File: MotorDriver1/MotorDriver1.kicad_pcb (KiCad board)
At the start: 2 copper layers, 74 parts, among them IC1 STM32C092RCT6, J1 GT-USB-7010ASV, J2 Conn_01x02, J3 Conn_01x02, Q1 IRLZ44NSTRLPBF, Q2 IRLZ44NSTRLPBF, Q3 IRLZ44NSTRLPBF, Q4 IRLZ44NSTRLPBF, SW1 K2-6639SP-C4SC-04, SW2 K2-6639SP-C4SC-04, SW3 K2-6639SP-C4SC-04, U1 TPS22916CNYFPR, U2 CH340X, U3 XIAO-ESP32-C5-DIP, U4 MCP2562FDT-H/SN, U5 MCP2562FDT-H/SN, U7 LMV358AIDR, Y1 48 MHz, Y2 32.768 kHz

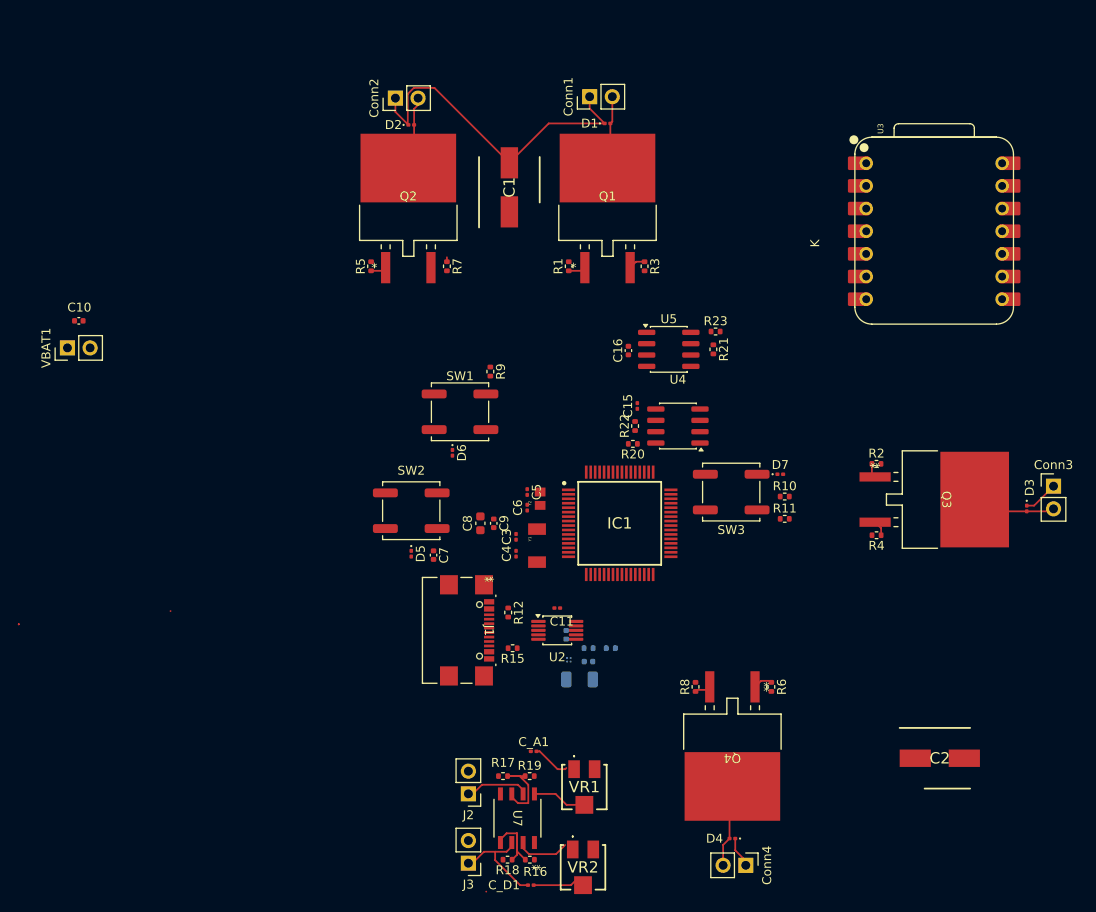
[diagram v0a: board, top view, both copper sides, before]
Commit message: Exported final JLCPCB files
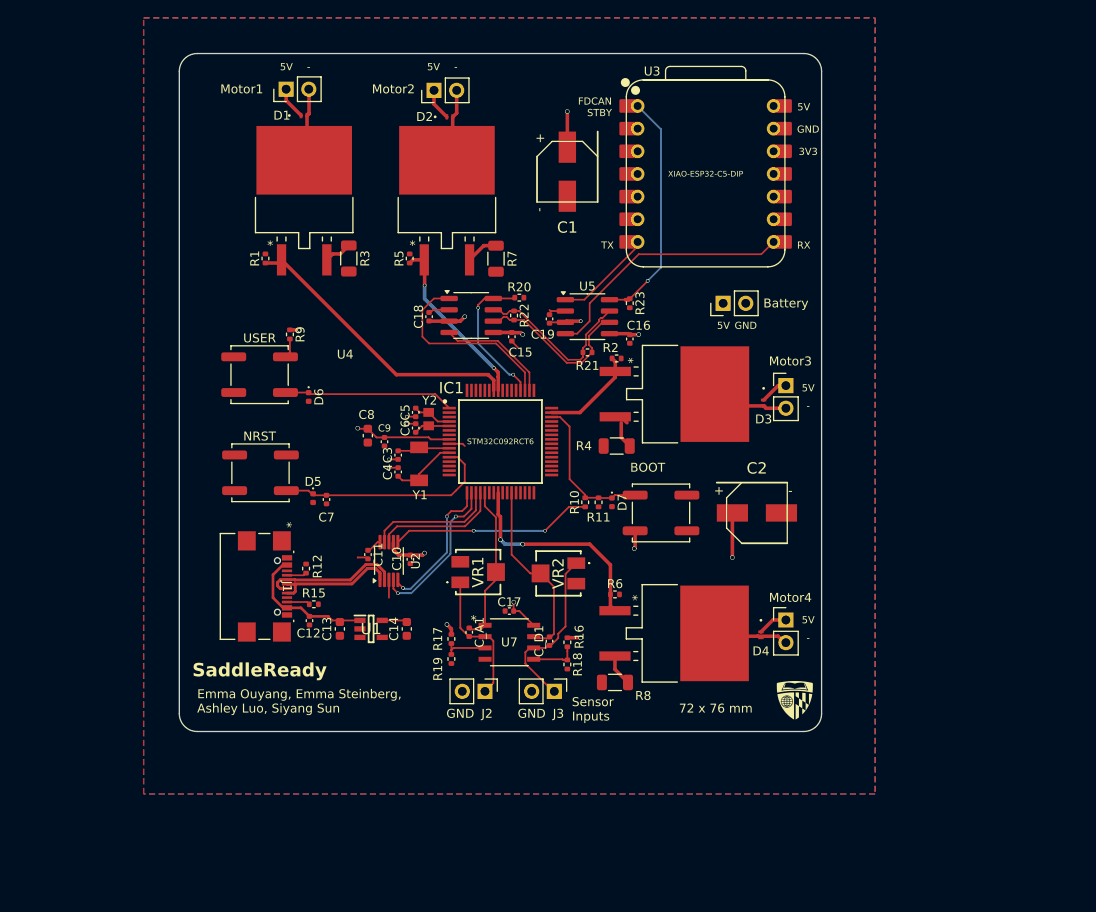
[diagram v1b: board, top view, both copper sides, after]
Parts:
- removed R13, R14: 10k, 1%, Resistor_SMD:R_0402_1005Metric
- added C17: 100 nF, Capacitor_SMD:C_0402_1005Metric, F.Cu at (153.0, 112.5)
- added C18: 100 nF, Capacitor_SMD:C_0402_1005Metric, F.Cu at (144.0, 79.5)
- added C19: 100 nF, Capacitor_SMD:C_0402_1005Metric, F.Cu at (157.5, 79.8)
- added G***: LOGO, LOGO, F.Cu at (185.0, 122.5)
- C10, C16: value 100nF -> 100 nF
- C11, C5, C6: footprint Capacitor_SMD:C_0201_0603Metric -> Capacitor_SMD:C_0402_1005Metric
- C12: value 100nF -> 100 nF; moved to F.Cu
- C13: value 100nF -> 1 uF; footprint Capacitor_SMD:C_0402_1005Metric -> Capacitor_SMD:C_0603_1608Metric; moved to F.Cu
- C14: value 10uF -> 1 uF; footprint Capacitor_SMD:C_1206_3216Metric -> Capacitor_SMD:C_0603_1608Metric; moved to F.Cu
- C15: value 100nF -> 100 nF; footprint Capacitor_SMD:C_0201_0603Metric -> Capacitor_SMD:C_0402_1005Metric
- C3, C4: value 8 pF -> 8 pF, 0.1%; footprint Capacitor_SMD:C_0201_0603Metric -> Capacitor_SMD:C_0402_1005Metric
- C_A1, C_D1: value 44nF -> 47 nF; footprint Capacitor_SMD:C_0201_0603Metric -> Capacitor_SMD:C_0402_1005Metric
- D1, D2, D3, D4: value Power_D -> SM5819L2-TP; footprint Diode_SMD:D_0201_0603Metric -> footprintLib:SDO_SM5819L2-TP_MCE
- D5, D6, D7: value ESDALC6V1-1U2 -> ESDALC6V1-1M2; footprint Diode_SMD:D_0201_0603Metric -> Diode_SMD:D_0402_1005Metric
- R1, R16, R17, R2, R5, R6: value 10000 -> 10k
- R18, R19: value 1800 -> 1.8k
- R3, R4, R7, R8: footprint Resistor_SMD:R_0402_1005Metric -> Resistor_SMD:R_1206_3216Metric
- U1: value TPS22916CNYFPR -> NCP361SNT1G; footprint footprintLib:TPS22916CNYFPR -> footprintLib:SOT95P275X110-5N; moved to F.Cu
- moved VBAT1 73.7 mm to (177.0, 78.0)
- moved C10 45.8 mm to (141.9, 106.7), turned to 90 degrees
- moved C2 34.3 mm to (180.8, 101.5)
- moved D1 34.0 mm to (130.0, 57.0)
- moved Conn1 34.0 mm to (128.0, 54.0)
- moved Q1 34.0 mm to (130.0, 65.1)
- moved R1 34.0 mm to (125.7, 73.0)
- moved R3 33.2 mm to (135.0, 73.0)
- moved VR2 33.1 mm to (158.5, 108.3), turned to 90 degrees
- moved Conn3 32.0 mm to (184.0, 87.2)
- moved D3 31.8 mm to (181.5, 89.2)
- moved Q3 31.4 mm to (172.9, 88.2)
- moved R2 31.4 mm to (165.0, 84.2)
- moved R4 30.8 mm to (165.0, 94.0)
- moved C12 28.8 mm to (130.6, 113.6)
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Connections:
- net /FDCAN/CANH renamed /FDCAN/CAN_P
- net /FDCAN/CANL renamed /FDCAN/CAN_N
- C1 pad 1: GND -> 5V
- C1 pad 2: 5V -> GND
- C13 pad 2: 5V_USB -> VBUS
- C2 pad 1: GND -> 5V
- C2 pad 2: 5V -> GND
- C_A1 pad 1: SensorAIn -> SensorAOut
- C_A1 pad 2: Net-(VR1-CCW) -> SensorAIn
- C_D1 pad 2: Net-(VR2-WIPER) -> SensorDOut
- SW1 pad 1: Net-(R9-Pad2) -> unconnected-(SW1-Pad1)
- SW1 pad 3: USER_BTN -> unconnected-(SW1-Pad3)
- SW2 pad 1: GND -> unconnected-(SW2-Pad1)
- SW2 pad 3: NRST -> unconnected-(SW2-Pad3)
- SW3 pad 1: 3V3 -> unconnected-(SW3-Pad1)
- SW3 pad 3: BOOT -> unconnected-(SW3-Pad3)
- VR1 pad A1: Net-(VR1-CCW) -> SensorAIn
- VR2 pad A1: SensorDOut -> SensorDIn
- VR2 pad B1: Net-(VR2-WIPER) -> SensorDOut
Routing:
- net 5V: track 45.8 -> 109.6 mm, vias 0 -> 4
- net 3V3: track 0.00 -> 31.8 mm, vias 0 -> 9
- net Motor1_PWM: track 1.95 -> 32.5 mm
- net FDCAN_RX_ESP: track 0.00 -> 28.8 mm
- net FDCAN_STBY_ESP: track 0.00 -> 27.0 mm, vias 0 -> 1
- net NRST: track 0.00 -> 24.9 mm
- net !DTR: track 0.00 -> 22.6 mm, vias 0 -> 2
- net Motor4_PWM: track 2.11 -> 24.2 mm, vias 0 -> 2
- net FDCAN_TX_STM: track 0.00 -> 21.9 mm
- net /FDCAN/CAN_P: track 0.00 -> 19.3 mm
- net USER_BTN: track 0.00 -> 19.1 mm
- net /FDCAN/CAN_N: track 0.00 -> 18.8 mm
- net Motor2_PWM: track 1.78 -> 20.4 mm, vias 0 -> 2
- net !RTS: track 0.00 -> 17.8 mm, vias 0 -> 2
- net BOOT: track 0.00 -> 16.9 mm
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- added copper zone on In2.Cu, net 3V3
- added copper zone on In2.Cu, net 5V
- added copper zone on B.Cu, net GND
- added copper zone on F.Cu, net GND
- added copper zone on In1.Cu, net GND
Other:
- board outline added: 72 x 76 mm
- copper layers 2 -> 4
- board text added: "+"
- board text added: "-"
- board text added: "3V3"
- board text added: "5V"
- board text added: "72 x 76 mm"
- board text added: "BOOT"
- board text added: "Battery"
- board text added: "Emma Ouyang, Emma Steinberg, Ashley Luo, Siyang Sun"
- board text added: "FDCAN STBY"
- board text added: "GND"
- board text added: "Motor1"
- board text added: "Motor2"
- board text added: "Motor3"
- board text added: "Motor4"
- board text added: "NRST"
- board text added: "RX"
- board text added: "STM32C092RCT6"
- board text added: "SaddleReady"
- board text added: "Sensor Inputs"
- board text added: "TX"
- board text added: "USER"
